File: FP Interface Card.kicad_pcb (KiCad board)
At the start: 4 copper layers, 90.2 x 101.1 mm, 66 parts, among them J1 T2M-105-01-X-D-TH-DS, J2 ZX62-AB-5PA(31), P1 Card Edge for HSEC8-160-01-S-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, Q1 Q_NMOS_GSD, Q2 Q_NMOS_GSD, Q3 Q_NMOS_GSD, Q4 Q_NMOS_GSD, Q5 BC847BM3T5G, Q6 BC847BM3T5G, Q7 BC847BM3T5G, Q8 BC847BM3T5G, SW1 SW_Push_SPST, U1 AP2161W

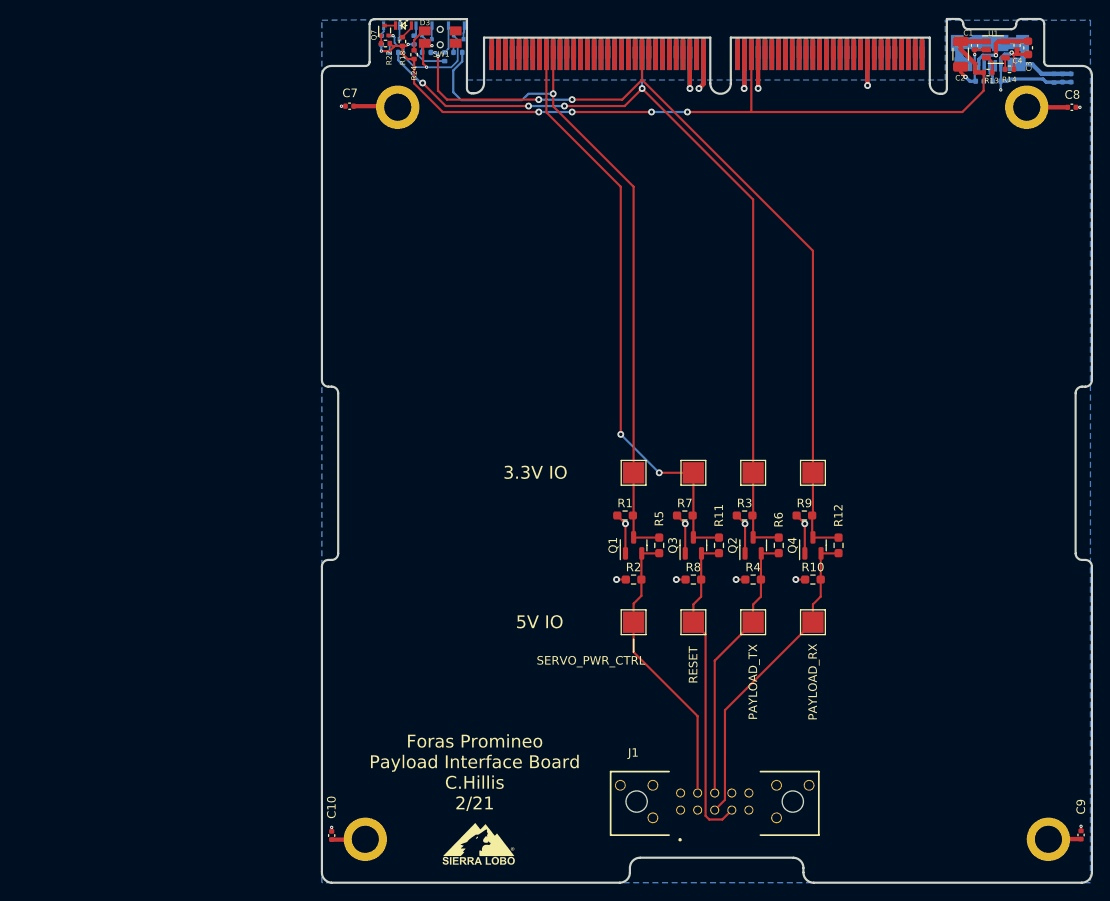
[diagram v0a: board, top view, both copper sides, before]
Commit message: majority of routing completed
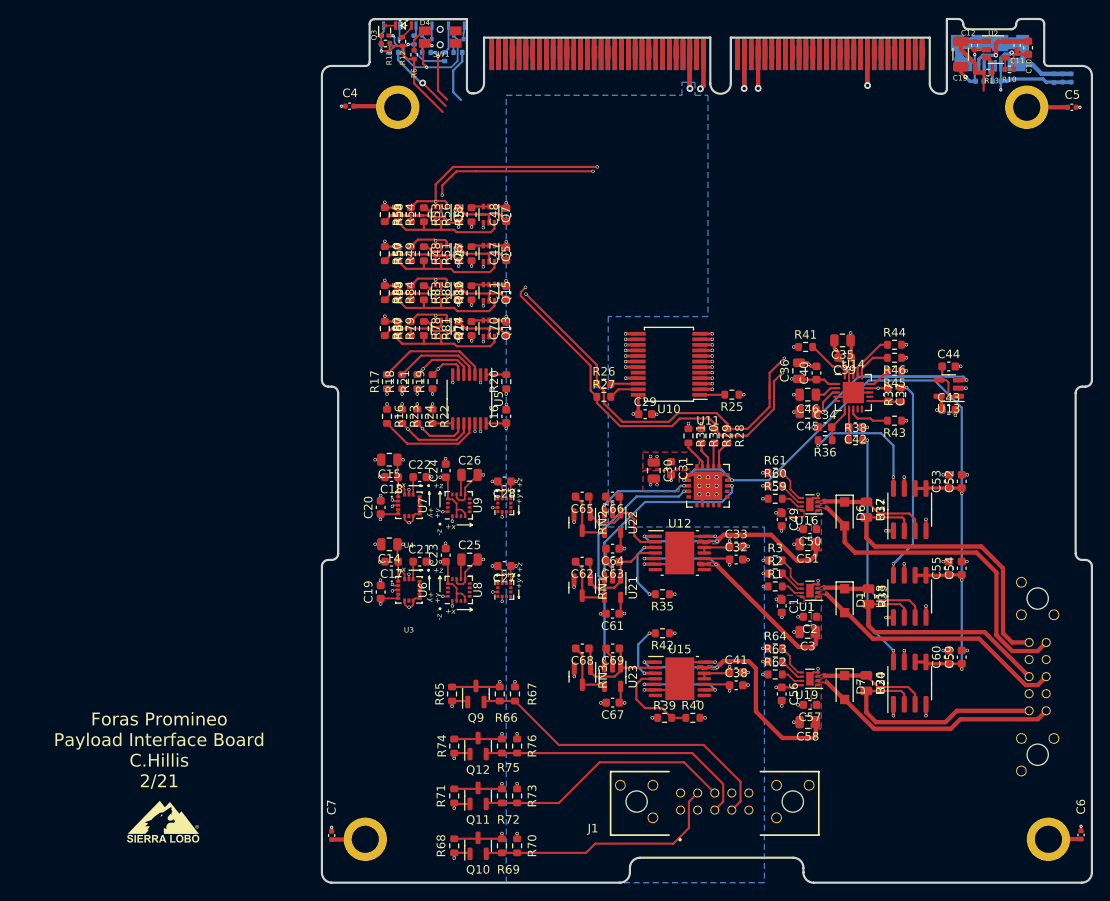
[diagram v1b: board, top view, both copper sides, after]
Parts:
- removed the Q1 at (36.5, -39.5)
- removed the Q2 at (50.5, -39.5)
- removed the Q3 at (43.5, -39.5)
- removed the Q4 at (57.5, -39.5)
- removed the R10 at (57.5, -35.5)
- removed the R11 at (46.5, -39.5)
- removed the R12 at (60.5, -39.5)
- removed the R4 at (50.5, -35.5)
- removed the R5 at (39.5, -39.5)
- removed the R6 at (53.5, -39.5)
- removed the R7 at (42.5, -43.0)
- removed the R8 at (43.5, -35.5)
- removed the R9 at (56.5, -43.0)
- removed TP1, TP2, TP3, TP4, TP5, TP6, TP7, TP8: TestPoint, TestPoint:TestPoint_Pad_2.5x2.5mm
- added C1: 0.1uF, Capacitor_SMD:C_0603_1608Metric, F.Cu at (53.8, -32.4)
- added C14: 2.2uF, Capacitor_SMD:C_0805_2012Metric, F.Cu at (7.90, -39.6)
- added C15: 2.2uF, Capacitor_SMD:C_0805_2012Metric, F.Cu at (7.90, -49.5)
- added C16: 0.1uF, Capacitor_SMD:C_0603_1608Metric, F.Cu at (21.6, -54.6)
- added C17: 0.1uF, Capacitor_SMD:C_0603_1608Metric, F.Cu at (8.15, -37.6)
- added C18: 0.1uF, Capacitor_SMD:C_0603_1608Metric, F.Cu at (8.15, -47.5)
- added C19: 10nF, Capacitor_SMD:C_0603_1608Metric, F.Cu at (6.88, -34.0)
- added C2: 0.1uF, Capacitor_SMD:C_0603_1608Metric, F.Cu at (57.1, -31.1)
- added C20: 10nF, Capacitor_SMD:C_0603_1608Metric, F.Cu at (6.88, -43.9)
- added C21: 0.47uF, Capacitor_SMD:C_0603_1608Metric, F.Cu at (11.5, -37.6)
- added C22: 0.47uF, Capacitor_SMD:C_0603_1608Metric, F.Cu at (11.5, -47.5)
- added C23: 1uF, Capacitor_SMD:C_0603_1608Metric, F.Cu at (14.5, -38.4)
- added C24: 1uF, Capacitor_SMD:C_0603_1608Metric, F.Cu at (14.5, -48.3)
- added C25: 10uF, Capacitor_SMD:C_0805_2012Metric, F.Cu at (17.3, -37.8)
- added C26: 10uF, Capacitor_SMD:C_0805_2012Metric, F.Cu at (17.3, -47.8)
- added C27: 1uF, Capacitor_SMD:C_0603_1608Metric, F.Cu at (21.4, -37.1)
- added C28: 1uF, Capacitor_SMD:C_0603_1608Metric, F.Cu at (21.4, -47.0)
- added C29: 0.1uF, Capacitor_SMD:C_0603_1608Metric, F.Cu at (37.9, -54.9)
- added C3: 4.7uF, Capacitor_SMD:C_0805_2012Metric, F.Cu at (56.9, -29.4)
- added C30: 10uF, Capacitor_SMD:C_0805_2012Metric, F.Cu at (38.9, -48.3)
- added C31: 0.1uF, Capacitor_SMD:C_0603_1608Metric, F.Cu at (40.9, -48.5)
- added C32: 0.1uF, Capacitor_SMD:C_0603_1608Metric, F.Cu at (48.5, -37.8)
- added C33: 0.1uF, Capacitor_SMD:C_0603_1608Metric, F.Cu at (48.5, -39.4)
- added C34: 560pF, Capacitor_SMD:C_0603_1608Metric, F.Cu at (58.9, -53.3)
- added C35: 10uF, Capacitor_SMD:C_0805_2012Metric, F.Cu at (61.0, -63.5)
- added C36: 10uF, Capacitor_SMD:C_0805_2012Metric, F.Cu at (55.9, -59.9)
- added C37: 560pF, Capacitor_SMD:C_0603_1608Metric, F.Cu at (66.3, -57.1)
- added C38: 0.1uF, Capacitor_SMD:C_0603_1608Metric, F.Cu at (48.5, -23.1)
- added C39: 0.1uF, Capacitor_SMD:C_0603_1608Metric, F.Cu at (61.2, -61.5)
- added C40: 0.1uF, Capacitor_SMD:C_0603_1608Metric, F.Cu at (57.9, -59.7)
- added C41: 0.1uF, Capacitor_SMD:C_0603_1608Metric, F.Cu at (48.5, -24.6)
- added C42: 560pF, Capacitor_SMD:C_0603_1608Metric, F.Cu at (62.5, -53.3)
- added C43: 0.1uF, Capacitor_SMD:C_0603_1608Metric, F.Cu at (73.4, -55.4)
- added C44: 0.1uF, Capacitor_SMD:C_0603_1608Metric, F.Cu at (73.4, -60.5)
- added C45: 2.2uF, Capacitor_SMD:C_0805_2012Metric, F.Cu at (56.9, -55.1)
- added C46: 2.2uF, Capacitor_SMD:C_0805_2012Metric, F.Cu at (56.9, -57.1)
- added C47: 10nF, Capacitor_SMD:C_0603_1608Metric, F.Cu at (21.6, -73.7)
- added C48: 10nF, Capacitor_SMD:C_0603_1608Metric, F.Cu at (21.6, -78.2)
- added C49: 0.1uF, Capacitor_SMD:C_0603_1608Metric, F.Cu at (53.8, -42.5)
- added C50: 0.1uF, Capacitor_SMD:C_0603_1608Metric, F.Cu at (57.1, -41.4)
- added C51: 4.7uF, Capacitor_SMD:C_0805_2012Metric, F.Cu at (56.9, -39.6)
- added C52: 1uF, Capacitor_SMD:C_0603_1608Metric, F.Cu at (74.9, -47.0)
- added C53: 0.1uF, Capacitor_SMD:C_0603_1608Metric, F.Cu at (73.4, -47.0)
- added C54: 1uF, Capacitor_SMD:C_0603_1608Metric, F.Cu at (74.9, -36.8)
- added C55: 0.1uF, Capacitor_SMD:C_0603_1608Metric, F.Cu at (73.4, -36.8)
- added C56: 0.1uF, Capacitor_SMD:C_0603_1608Metric, F.Cu at (53.8, -22.1)
- added C57: 0.1uF, Capacitor_SMD:C_0603_1608Metric, F.Cu at (57.1, -20.8)
- added C58: 4.7uF, Capacitor_SMD:C_0805_2012Metric, F.Cu at (56.9, -18.8)
- added C59: 1uF, Capacitor_SMD:C_0603_1608Metric, F.Cu at (74.9, -26.4)
- added C60: 0.1uF, Capacitor_SMD:C_0603_1608Metric, F.Cu at (73.4, -26.4)
- added C61: 0.1uF, Capacitor_SMD:C_0603_1608Metric, F.Cu at (34.0, -31.5)
- added C62: 0.1uF, Capacitor_SMD:C_0603_1608Metric, F.Cu at (30.5, -37.6)
- added C63: 0.1uF, Capacitor_SMD:C_0603_1608Metric, F.Cu at (34.0, -37.6)
- added C64: 0.1uF, Capacitor_SMD:C_0603_1608Metric, F.Cu at (34.0, -39.1)
- added C65: 0.1uF, Capacitor_SMD:C_0603_1608Metric, F.Cu at (30.5, -45.2)
- added C66: 0.1uF, Capacitor_SMD:C_0603_1608Metric, F.Cu at (34.0, -45.2)
- added C67: 0.1uF, Capacitor_SMD:C_0603_1608Metric, F.Cu at (34.1, -21.1)
- added C68: 0.1uF, Capacitor_SMD:C_0603_1608Metric, F.Cu at (30.5, -27.4)
- added C69: 0.1uF, Capacitor_SMD:C_0603_1608Metric, F.Cu at (34.1, -27.4)
- added C70: 10nF, Capacitor_SMD:C_0603_1608Metric, F.Cu at (21.6, -64.9)
- added C71: 10nF, Capacitor_SMD:C_0603_1608Metric, F.Cu at (21.6, -69.1)
- added D1: TPSMF4L6.0A, Diode_SMD:D_SOD-123F, F.Cu at (61.2, -33.0)
- added D6: TPSMF4L6.0A, Diode_SMD:D_SOD-123F, F.Cu at (61.2, -43.2)
- added D7: TPSMF4L6.0A, Diode_SMD:D_SOD-123F, F.Cu at (61.2, -22.9)
- added J2: T2M-105-01-X-D-TH-DS, payload-interface-board:SAMTEC_T2M-105-01-X-D-TH-DS, B.Cu at (83.8, -24.1)
- added Q10: Q_NMOS_GSD, Package_TO_SOT_SMD:SOT-23, F.Cu at (18.3, -4.32)
- added Q11: Q_NMOS_GSD, Package_TO_SOT_SMD:SOT-23, F.Cu at (18.3, -10.2)
- added Q12: Q_NMOS_GSD, Package_TO_SOT_SMD:SOT-23, F.Cu at (18.3, -16.0)
- added Q13: BSS138DWQ-7, Package_TO_SOT_SMD:SOT-363_SC-70-6, F.Cu at (19.6, -64.9)
- added Q14: MMDT5551-7-F, Package_TO_SOT_SMD:SOT-363_SC-70-6, F.Cu at (14.0, -64.9)
- added Q15: BSS138DWQ-7, Package_TO_SOT_SMD:SOT-363_SC-70-6, F.Cu at (19.6, -69.1)
- added Q16: MMDT5551-7-F, Package_TO_SOT_SMD:SOT-363_SC-70-6, F.Cu at (14.0, -69.1)
- added Q5: BSS138DWQ-7, Package_TO_SOT_SMD:SOT-363_SC-70-6, F.Cu at (19.6, -73.7)
- added Q6: MMDT5551-7-F, Package_TO_SOT_SMD:SOT-363_SC-70-6, F.Cu at (14.0, -73.7)
- added Q7: BSS138DWQ-7, Package_TO_SOT_SMD:SOT-363_SC-70-6, F.Cu at (19.6, -78.2)
- added Q8: MMDT5551-7-F, Package_TO_SOT_SMD:SOT-363_SC-70-6, F.Cu at (14.0, -78.2)
- added Q9: Q_NMOS_GSD, Package_TO_SOT_SMD:SOT-23, F.Cu at (18.0, -22.1)
- added R16: 100k, Resistor_SMD:R_0603_1608Metric, F.Cu at (7.62, -54.6)
- added R17: 100k, Resistor_SMD:R_0603_1608Metric, F.Cu at (7.62, -58.7)
- added R18: 100k, Resistor_SMD:R_0603_1608Metric, F.Cu at (9.40, -58.7)
- added R19: 10k, Resistor_SMD:R_0603_1608Metric, F.Cu at (13.0, -58.7)
- added R20: 100k, Resistor_SMD:R_0603_1608Metric, F.Cu at (21.6, -58.7)
- added R21: 10k, Resistor_SMD:R_0603_1608Metric, F.Cu at (11.2, -58.7)
- added R22: 100k, Resistor_SMD:R_0603_1608Metric, F.Cu at (13.0, -54.6)
- added R23: 10k, Resistor_SMD:R_0603_1608Metric, F.Cu at (9.40, -54.6)
- added R24: 10k, Resistor_SMD:R_0603_1608Metric, F.Cu at (11.2, -54.6)
- added R25: 100k, Resistor_SMD:R_0603_1608Metric, F.Cu at (48.0, -57.1)
- added R26: 51, Resistor_SMD:R_0603_1608Metric, F.Cu at (33.0, -58.4)
- added R27: 51, Resistor_SMD:R_0603_1608Metric, F.Cu at (33.0, -56.9)
- added R28: 51, Resistor_SMD:R_0603_1608Metric, F.Cu at (47.5, -52.3)
- added R29: 51, Resistor_SMD:R_0603_1608Metric, F.Cu at (46.0, -52.3)
- added R30: 100, Resistor_SMD:R_0603_1608Metric, F.Cu at (44.5, -52.3)
- added R31: 100, Resistor_SMD:R_0603_1608Metric, F.Cu at (42.9, -52.3)
- added R32: 200mR, Resistor_SMD:R_0805_2012Metric, F.Cu at (63.8, -43.7)
- added R33: 200mR, Resistor_SMD:R_0805_2012Metric, F.Cu at (64.0, -33.5)
- added R34: 91mR, Resistor_SMD:R_0805_2012Metric, F.Cu at (63.8, -23.4)
- added R35: 100k, Resistor_SMD:R_0603_1608Metric, F.Cu at (39.9, -33.8)
- added R36: 33, Resistor_SMD:R_0603_1608Metric, F.Cu at (58.9, -51.8)
- added R37: 33, Resistor_SMD:R_0603_1608Metric, F.Cu at (67.8, -57.1)
- added R38: 33, Resistor_SMD:R_0603_1608Metric, F.Cu at (62.5, -51.8)
- added R39: 100k, Resistor_SMD:R_0603_1608Metric, F.Cu at (40.1, -19.3)
- added R40: 100k, Resistor_SMD:R_0603_1608Metric, F.Cu at (43.4, -19.3)
- added R41: 100, Resistor_SMD:R_0603_1608Metric, F.Cu at (56.6, -62.7)
- added R42: 100k, Resistor_SMD:R_0603_1608Metric, F.Cu at (39.9, -29.2)
- added R43: 100, Resistor_SMD:R_0603_1608Metric, F.Cu at (67.1, -54.1)
- added R44: 100, Resistor_SMD:R_0603_1608Metric, F.Cu at (67.1, -63.0)
- added R45: 51, Resistor_SMD:R_0603_1608Metric, F.Cu at (67.1, -59.9)
- added R46: 51, Resistor_SMD:R_0603_1608Metric, F.Cu at (67.1, -61.5)
- added R47: 100k, Resistor_SMD:R_0603_1608Metric, F.Cu at (17.5, -73.7)
- added R48: 680, Resistor_SMD:R_0603_1608Metric, F.Cu at (11.9, -73.7)
- added R49: 10k, Resistor_SMD:R_0603_1608Metric, F.Cu at (8.89, -73.7)
- added R50: 10k, Resistor_SMD:R_0603_1608Metric, F.Cu at (7.37, -73.7)
- added R51: 200K, Resistor_SMD:R_0603_1608Metric, F.Cu at (16.0, -73.7)
- added R52: 100k, Resistor_SMD:R_0603_1608Metric, F.Cu at (17.5, -78.2)
- added R53: 680, Resistor_SMD:R_0603_1608Metric, F.Cu at (11.9, -78.2)
- added R54: 10k, Resistor_SMD:R_0603_1608Metric, F.Cu at (8.89, -78.2)
- added R55: 10k, Resistor_SMD:R_0603_1608Metric, F.Cu at (7.37, -78.2)
- added R56: 200K, Resistor_SMD:R_0603_1608Metric, F.Cu at (16.0, -78.2)
- added R57: 0, Resistor_SMD:R_0603_1608Metric, F.Cu at (10.4, -73.7)
- added R58: 0, Resistor_SMD:R_0603_1608Metric, F.Cu at (10.4, -78.2)
- added R59: 100, Resistor_SMD:R_0603_1608Metric, F.Cu at (53.1, -45.0)
- added R60: 100, Resistor_SMD:R_0603_1608Metric, F.Cu at (53.1, -46.5)
- added R61: 100, Resistor_SMD:R_0603_1608Metric, F.Cu at (53.1, -48.0)
- added R62: 100, Resistor_SMD:R_0603_1608Metric, F.Cu at (53.1, -24.4)
- added R63: 100, Resistor_SMD:R_0603_1608Metric, F.Cu at (53.1, -25.9)
- added R64: 100, Resistor_SMD:R_0603_1608Metric, F.Cu at (53.1, -27.4)
- added R65: 10k, Resistor_SMD:R_0603_1608Metric, F.Cu at (15.2, -22.1)
- added R66: DNP, Resistor_SMD:R_0603_1608Metric, F.Cu at (20.8, -22.1)
- added R67: 10k, Resistor_SMD:R_0603_1608Metric, F.Cu at (22.6, -22.1)
- added R68: 10k, Resistor_SMD:R_0603_1608Metric, F.Cu at (15.5, -4.32)
- added R69: DNP, Resistor_SMD:R_0603_1608Metric, F.Cu at (21.1, -4.32)
- added R70: 10k, Resistor_SMD:R_0603_1608Metric, F.Cu at (22.9, -4.32)
- added R71: 10k, Resistor_SMD:R_0603_1608Metric, F.Cu at (15.5, -10.2)
- added R72: DNP, Resistor_SMD:R_0603_1608Metric, F.Cu at (21.1, -10.2)
- added R73: 10k, Resistor_SMD:R_0603_1608Metric, F.Cu at (22.9, -10.2)
- added R74: 10k, Resistor_SMD:R_0603_1608Metric, F.Cu at (15.5, -16.0)
- added R75: DNP, Resistor_SMD:R_0603_1608Metric, F.Cu at (21.1, -16.0)
- added R76: 10k, Resistor_SMD:R_0603_1608Metric, F.Cu at (22.9, -16.0)
- added R77: 100k, Resistor_SMD:R_0603_1608Metric, F.Cu at (17.5, -64.9)
- added R78: 680, Resistor_SMD:R_0603_1608Metric, F.Cu at (11.9, -64.9)
- added R79: 10k, Resistor_SMD:R_0603_1608Metric, F.Cu at (8.89, -64.9)
- added R80: 10k, Resistor_SMD:R_0603_1608Metric, F.Cu at (7.37, -64.9)
- added R81: 200K, Resistor_SMD:R_0603_1608Metric, F.Cu at (16.0, -64.9)
- added R82: 100k, Resistor_SMD:R_0603_1608Metric, F.Cu at (17.5, -69.1)
- added R83: 680, Resistor_SMD:R_0603_1608Metric, F.Cu at (11.9, -69.1)
- added R84: 10k, Resistor_SMD:R_0603_1608Metric, F.Cu at (8.89, -69.1)
- added R85: 10k, Resistor_SMD:R_0603_1608Metric, F.Cu at (7.37, -69.1)
- added R86: 200K, Resistor_SMD:R_0603_1608Metric, F.Cu at (16.0, -69.1)
- added R87: 0, Resistor_SMD:R_0603_1608Metric, F.Cu at (10.4, -64.9)
- added R88: 0, Resistor_SMD:R_0603_1608Metric, F.Cu at (10.4, -69.1)
- added RN1: MAX5490GC01000+T, Package_TO_SOT_SMD:SOT-23, F.Cu at (30.5, -34.5)
- added RN2: MAX5490GC01000+T, Package_TO_SOT_SMD:SOT-23, F.Cu at (30.5, -42.2)
- added RN3: MAX5490GC01000+T, Package_TO_SOT_SMD:SOT-23, F.Cu at (30.5, -24.1)
- added U1: DRV8838DSGT, Package_SON:WSON-8-1EP_2x2mm_P0.5mm_EP0.9x1.6mm, F.Cu at (57.1, -34.2)
- added U10: MAX7311AAG+, Package_SO:SSOP-24_5.3x8.2mm_P0.65mm, F.Cu at (40.6, -60.7)
- added U11: MCP47FVB24-E/MQ, payload-interface-board:MCP47FVB24EMQ, F.Cu at (45.2, -46.5)
- added U12: ALM2402QPWPRQ1, Package_SO:HTSSOP-14-1EP_4.4x5mm_P0.65mm_EP3.4x5mm_Mask3x3.1mm, F.Cu at (41.9, -38.6)
- added U13: OPA340MDBVTEP, Package_TO_SOT_SMD:SOT-23-5, F.Cu at (73.4, -57.9)
- added U14: AD7091R-5BCPZ-RL7, Package_DFN_QFN:QFN-20-1EP_4x4mm_P0.5mm_EP2.5x2.5mm, F.Cu at (62.2, -57.4)
- added U15: ALM2402QPWPRQ1, Package_SO:HTSSOP-14-1EP_4.4x5mm_P0.65mm_EP3.4x5mm_Mask3x3.1mm, F.Cu at (41.9, -23.9)
- added U16: DRV8838DSGT, Package_SON:WSON-8-1EP_2x2mm_P0.5mm_EP0.9x1.6mm, F.Cu at (57.1, -44.3)
- added U17: INA240A3EDRQ1, Package_SO:SOIC-8_3.9x4.9mm_P1.27mm, F.Cu at (68.8, -43.7)
- added U18: INA240A3EDRQ1, Package_SO:SOIC-8_3.9x4.9mm_P1.27mm, F.Cu at (68.8, -33.5)
- added U19: DRV8838DSGT, Package_SON:WSON-8-1EP_2x2mm_P0.5mm_EP0.9x1.6mm, F.Cu at (57.1, -23.9)
- added U20: INA240A3EDRQ1, Package_SO:SOIC-8_3.9x4.9mm_P1.27mm, F.Cu at (68.8, -23.4)
- added U21: OPA340MDBVTEP, Package_TO_SOT_SMD:SOT-23-5, F.Cu at (34.0, -34.5)
- added U22: OPA340MDBVTEP, Package_TO_SOT_SMD:SOT-23-5, F.Cu at (34.0, -42.2)
- added U23: OPA340MDBVTEP, Package_TO_SOT_SMD:SOT-23-5, F.Cu at (34.0, -24.1)
- added U3: IAM-20380, payload-interface-board:IAM-20380, F.Cu at (10.2, -34.3)
- added U4: IAM-20380, payload-interface-board:IAM-20380, F.Cu at (10.2, -44.2)
- added U5: PCA9543APW,118, Package_SO:TSSOP-14_4.4x5mm_P0.65mm, F.Cu at (17.3, -56.6)
- added U6: MMC5983MA, payload-interface-board:MMC5983MA, F.Cu at (16.0, -34.3)
- added U7: MMC5983MA, payload-interface-board:MMC5983MA, F.Cu at (16.0, -44.2)
- added U8: MXC6655XA, payload-interface-board:MXC6655XA, F.Cu at (21.4, -34.3)
- added U9: MXC6655XA, payload-interface-board:MXC6655XA, F.Cu at (21.4, -44.2)
- R1, R2, R3: value 10k -> 100; footprint Resistor_SMD:R_0603_1608Metric_Pad0.98x0.95mm_HandSolder -> Resistor_SMD:R_0603_1608Metric
- moved G*** 37.0 mm to (-18.6, -7.14)
- moved R1 19.4 mm to (53.1, -34.7)
- moved R2 16.6 mm to (53.1, -36.2)
- moved R3 6.36 mm to (53.1, -37.7)
- renumbered C3 to C10, C4 to C11, C1 to C12, C2 to C13, C7 to C4, C8 to C5, C9 to C6, C10 to C7, C5 to C8, C6 to C9, D1 to D2, D2 to D3, D3 to D4, D4 to D5, J2 to J3, Q5 to Q1, Q6 to Q2, Q7 to Q3, Q8 to Q4, R14 to R10, R22 to R11, R18 to R12, R23 to R14, R19 to R15, R20 to R4, R15 to R5, R24 to R6, R16 to R7, R21 to R8, R17 to R9, U1 to U2
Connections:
- R1 pad 1: +3V3 -> /Magnetotorquer Drivers/~{DRV_SLP_Y}
- R1 pad 2: /H2-6 -> Net-(R1-Pad2)
- R2 pad 1: +5V -> /Magnetotorquer Drivers/DRV_PH_Y
- R2 pad 2: /SERVO_PWR_CTRL -> Net-(R2-Pad2)
- R3 pad 1: +3V3 -> /Magnetotorquer Drivers/DRV_EN_Y
- R3 pad 2: /H1-19 -> Net-(R3-Pad2)
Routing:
- net GND: track 69.8 -> 205.6 mm, vias 14 -> 106
- net /Magnetotorquer Drivers/2.5V_Vref: track 0.00 -> 98.9 mm, vias 0 -> 6
- net /SDA_Magnetotorquers: track 0.00 -> 87.5 mm, vias 0 -> 4
- net /SCL_Magnetotorquers: track 0.00 -> 85.7 mm, vias 0 -> 4
- net /5V_USB: track 102.2 -> 31.5 mm, vias 6 -> 2
- net +3V3: track 26.9 -> 97.5 mm, vias 5 -> 41
- net /Magnetotorquer Drivers/DRV_EN_Z: track 0.00 -> 61.5 mm, vias 0 -> 2
- net /Magnetotorquer Drivers/~{DRV_SLP_Z}: track 0.00 -> 58.8 mm, vias 0 -> 2
- net /Magnetotorquer Drivers/DRV_PH_Z: track 0.00 -> 57.5 mm, vias 0 -> 2
- net /Magnetotorquer Drivers/ADC_ALERT/BUSY: track 0.00 -> 54.6 mm, vias 0 -> 2
- net /Magnetotorquer Drivers/~{DRV_SLP_Y}: track 0.00 -> 53.7 mm, vias 0 -> 2
- net /IMU/SCL_IMU2: track 0.00 -> 53.6 mm, vias 0 -> 4
- net /Magnetotorquer Drivers/DRV_EN_Y: track 0.00 -> 53.0 mm, vias 0 -> 2
- net /IMU/SDA_IMU2: track 0.00 -> 48.3 mm, vias 0 -> 4
- net /Magnetotorquer Drivers/~{AMP_SHDN_Z}: track 0.00 -> 46.2 mm, vias 0 -> 3
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- added copper zone on F.Cu, net +3V3
- added copper zone on In3.Cu, net +3V3
- added copper zone on B.Cu, net +5V
- added copper zone on F.Cu, net /Magnetotorquer Drivers/Full Bridge 1/OUT2
- added copper zone on F.Cu, net /Magnetotorquer Drivers/Full Bridge 2/OUT2
- added copper zone on F.Cu, net /Magnetotorquer Drivers/Full Bridge 3/OUT2
- added copper zone on F.Cu, net /Magnetotorquer Drivers/X_Drive
- added copper zone on F.Cu, net /Magnetotorquer Drivers/Y_Drive
- added copper zone on F.Cu, net /Magnetotorquer Drivers/Z_drive
- added copper zone on F.Cu, net /X+
- added copper zone on F.Cu, net /Y+
- added copper zone on F.Cu, net /Z+
- added copper zone on F.Cu, net GND
- added copper zone on In1.Cu, net GND
- added copper zone on In4.Cu, net GND
- removed copper zone on B.Cu, net +3V3
- removed copper zone on In1.Cu, net +5V
- removed copper zone on In2.Cu, net GND
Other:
- copper layers 4 -> 6
- board text removed: "3.3V IO"
- board text removed: "5V IO"
- board text removed: "PAYLOAD_RX"
- board text removed: "PAYLOAD_TX"
- board text removed: "RESET"
- board text removed: "SERVO_PWR_CTRL"

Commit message: updated board
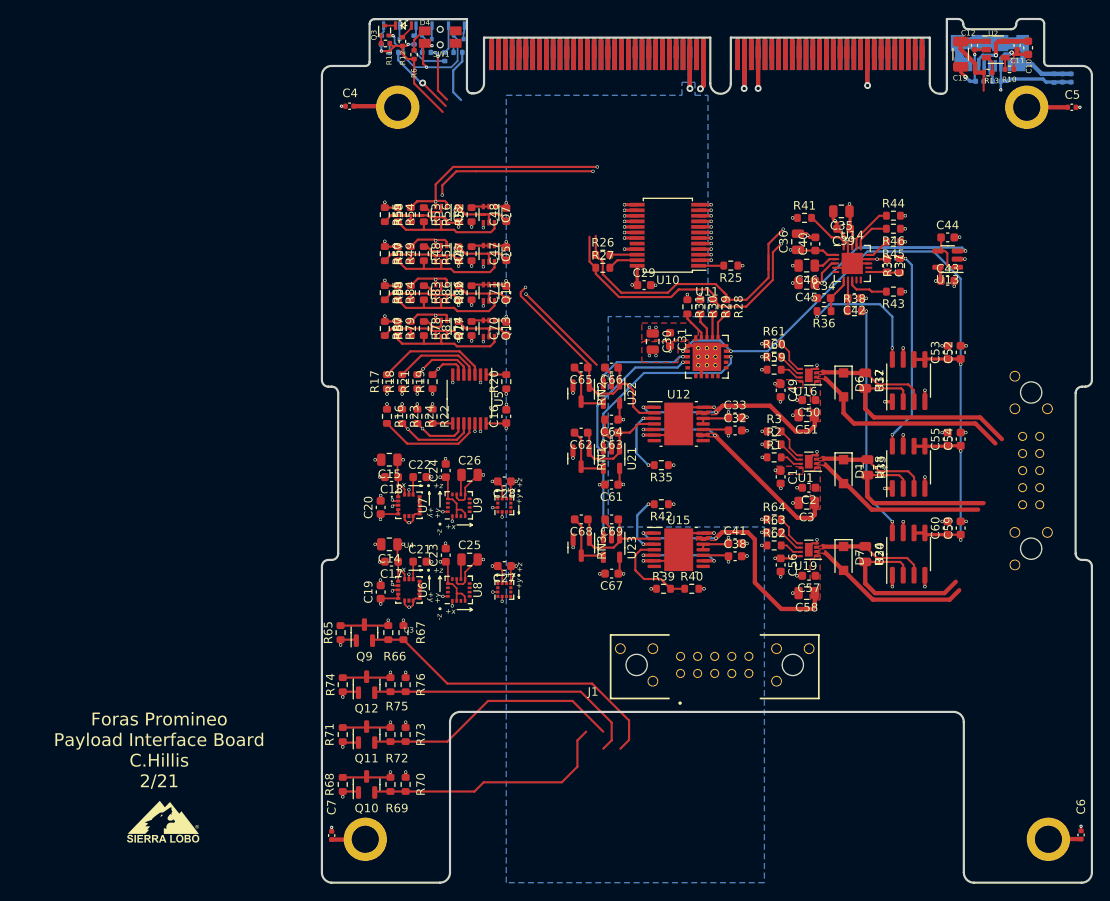
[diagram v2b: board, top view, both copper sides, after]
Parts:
- moved J2 24.1 mm to (83.1, -48.3)
- moved J1 16.0 mm to (46.0, -25.5)
- moved C1 15.1 mm to (53.7, -47.5)
- moved C29 15.1 mm to (37.7, -70.0)
- moved C32 15.1 mm to (48.4, -53.0)
- moved C37 15.1 mm to (66.2, -72.3)
- moved C46 15.1 mm to (56.8, -72.3)
- moved R25 15.1 mm to (47.9, -72.3)
- moved R35 15.1 mm to (39.8, -48.9)
- moved R37 15.1 mm to (67.7, -72.3)
- moved R43 15.1 mm to (66.9, -69.2)
- moved R44 15.1 mm to (66.9, -78.1)
- moved U13 15.1 mm to (73.3, -73.0)
- moved C3 15.1 mm to (56.8, -44.5)
- moved C57 15.1 mm to (57.0, -35.9)
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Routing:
- net /X+: track 38.7 -> 24.3 mm
- net /X-: track 36.9 -> 25.7 mm
- net /Y+: track 30.5 -> 20.0 mm
- net /Z+: track 28.9 -> 18.4 mm
- net /Z-: track 28.4 -> 19.9 mm
- net /Y-: track 29.3 -> 21.9 mm
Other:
- outline, holes or cut-outs redrawn
